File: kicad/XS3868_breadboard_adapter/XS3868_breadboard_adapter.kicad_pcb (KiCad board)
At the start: 2 copper layers, 26.4 x 31.5 mm, 12 parts, among them J1 SCJ368R1NUS0B00G, P1 CONN_01X12, P2 CONN_01X12, U1 XS3868

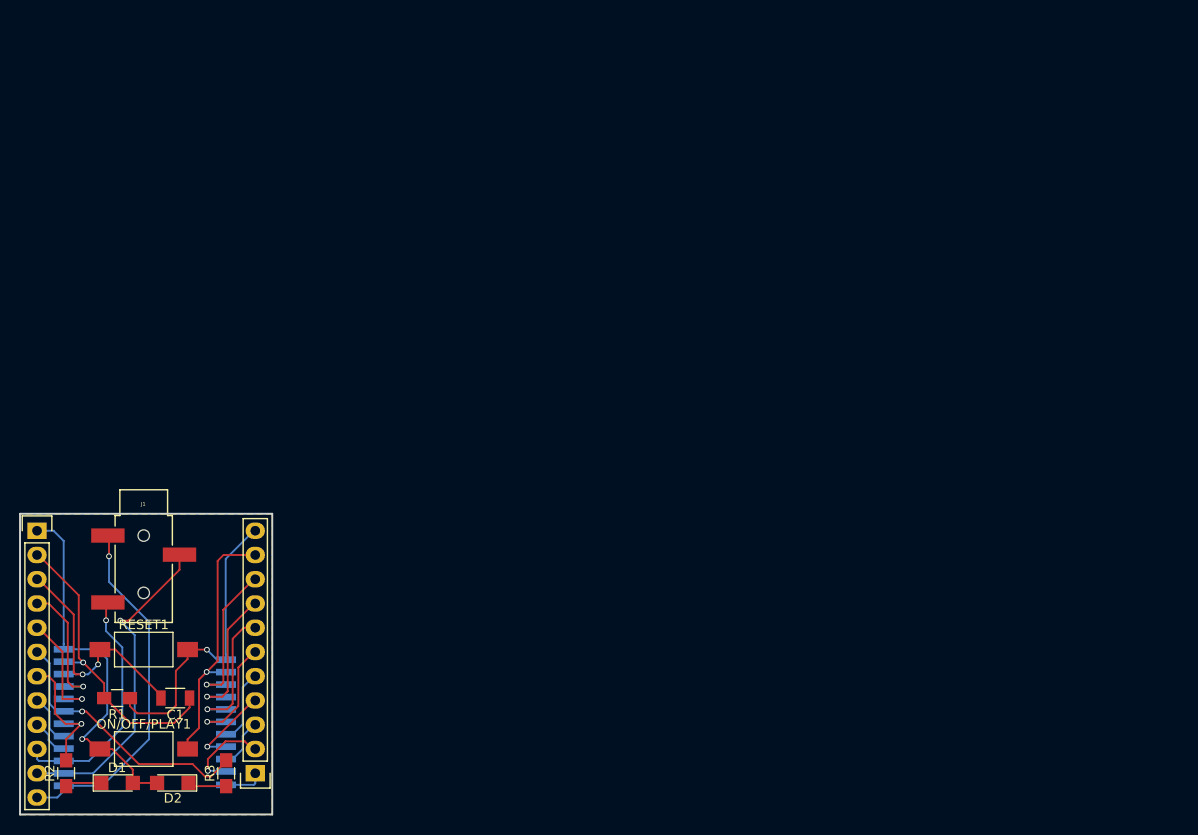
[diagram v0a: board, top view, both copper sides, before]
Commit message: update
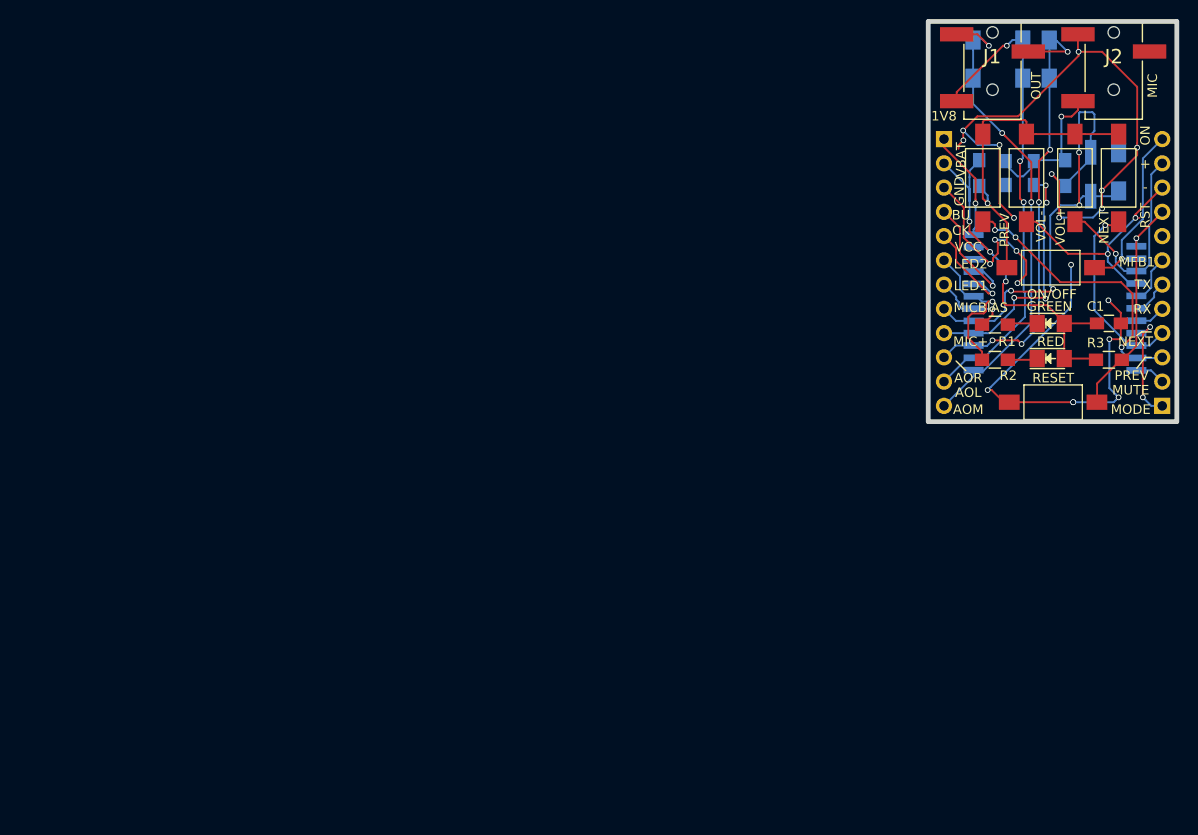
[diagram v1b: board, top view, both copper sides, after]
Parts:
- removed D1, D2: LED, LEDs:LED_1206
- removed ON/OFF/PLAY1: ON/OFF, Buttons_Switches_SMD:SW_SPST_FSMSM
- removed RESET1: 1, Buttons_Switches_SMD:SW_SPST_FSMSM
- added C2: 4u7, Capacitors_SMD.pretty:C_1206_HandSoldering, B.Cu at (164.1, 84.3)
- added C3: 2u2/6.5V, Capacitors_SMD.pretty:C_0805_HandSoldering, B.Cu at (155.2, 84.5)
- added C4: 220p/optional, Capacitors_SMD.pretty:C_0805_HandSoldering, B.Cu at (152.3, 84.5)
- added C5: 10uF, Capacitors_SMD.pretty:C_1206_HandSoldering, B.Cu at (148.8, 72.5)
- added C6: 10uF, Capacitors_SMD.pretty:C_1206_HandSoldering, B.Cu at (154.1, 72.5)
- added C7: 10uF, Capacitors_SMD.pretty:C_1206_HandSoldering, B.Cu at (156.8, 72.5)
- added GREEN: GREEN, LEDs:LED-1206, F.Cu at (157.0, 100.2)
- added J2: MIC, jacks:3.5mm_stereo_jack_PJ320B, F.Cu at (163.6, 69.7)
- added L1: 15n, Choke_SMD.pretty:Choke_SMD_1206_Handsoldering, B.Cu at (161.2, 84.6)
- added R4: 2k2, Resistors_SMD:R_0805_HandSoldering, B.Cu at (158.5, 84.5)
- added R5: 2k, Resistors_SMD:R_0805_HandSoldering, B.Cu at (149.5, 84.5)
- added RED: RED, LEDs:LED-1206, F.Cu at (157.0, 103.9)
- added SW1: PREV, Buttons_Switches_SMD:SW_SPST_FSMSM, F.Cu at (149.9, 85.0)
- added SW2: NEXT, Buttons_Switches_SMD:SW_SPST_FSMSM, F.Cu at (164.1, 85.0)
- added SW3: VOL-, Buttons_Switches_SMD:SW_SPST_FSMSM, F.Cu at (154.4, 85.0)
- added SW4: VOL+, Buttons_Switches_SMD:SW_SPST_FSMSM, F.Cu at (159.5, 85.0)
- added SW5: ON/OFF, Buttons_Switches_SMD:SW_SPST_FSMSM, F.Cu at (157.0, 94.4)
- added SW6: RESET, Buttons_Switches_SMD:SW_SPST_FSMSM, F.Cu at (157.2, 108.5)
- C1: footprint Capacitors_SMD:C_1206 -> Capacitors_SMD.pretty:C_0805_HandSoldering
- J1: value SCJ368R1NUS0B00G -> OUT
- P1: footprint Pin_Headers.pretty:Pin_Header_Straight_1x12 -> Pin_Headers:Pin_Header_Straight_1x12_Pitch2.54mm; moved to B.Cu
- P2: footprint Pin_Headers.pretty:Pin_Header_Straight_1x11 -> Pin_Headers:Pin_Header_Straight_1x12_Pitch2.54mm; moved to B.Cu
- R1: value 10k -> 470
- R3: value 470 -> 10k
- U1: footprint modules:XS3868 -> bluetooth:XS3868
- moved R2 106.5 mm to (151.1, 104.0), turned to 180 degrees
- moved C1 105.4 mm to (163.1, 100.2)
- moved U1 104.4 mm to (148.9, 89.6)
- moved P1 103.5 mm to (145.8, 80.9), turned to 180 degrees
- moved J1 103.3 mm to (150.9, 69.7)
- moved P2 102.5 mm to (168.7, 108.8), turned to 0 degrees
- moved R3 102.1 mm to (163.1, 104.0), turned to 180 degrees
- moved R1 99.9 mm to (151.1, 100.3)
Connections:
- net Net-(D1-Pad2) renamed /1V8
- net Net-(J1-Pad1) renamed /AOM
- net Net-(J1-Pad2) renamed /AOL
- net Net-(P1-Pad4) renamed /VBUCK
- net Net-(P1-Pad5) renamed /VCC
- net Net-(P1-Pad8) renamed /MICBIAS
- net Net-(P1-Pad9) renamed /MIC+
- net Net-(P2-Pad5) renamed /UART_RX
- net Net-(P2-Pad6) renamed /UART_TX
- net Net-(P2-Pad7) renamed /MFB1
- C1 pad 1: Net-(C1-Pad1) -> GND
- C1 pad 2: GND -> /VBAT
- P1 pad 10: Net-(J1-Pad5) -> /AOR
- P1 pad 2: Net-(C1-Pad1) -> /VBAT
- P1 pad 6: Net-(P1-Pad6) -> /LED2
- P1 pad 7: Net-(P1-Pad7) -> /LED1
- P2 pad 1: Net-(P2-Pad1) -> /MODE
- P2 pad 10: Net-(ON/OFF/PLAY1-Pad2) -> /VOL-
- P2 pad 11: Net-(P2-Pad11) -> /VOL+
- P2 pad 2: Net-(P2-Pad2) -> /MUTE
- P2 pad 3: Net-(P2-Pad3) -> /PREVIOUS
- P2 pad 4: Net-(P2-Pad4) -> /NEXT
- P2 pad 8: Net-(P2-Pad8) -> (no net)
- P2 pad 9: Net-(P2-Pad9) -> /RESET
- R1 pad 1: Net-(P2-Pad11) -> Net-(DG1-Pad1)
- R1 pad 2: Net-(C1-Pad1) -> /LED1
- R2 pad 2: Net-(P1-Pad7) -> /LED2
- R3 pad 1: Net-(D2-Pad1) -> /RESET
- R3 pad 2: Net-(P1-Pad6) -> /VBAT
- U1 pad 11: Net-(C1-Pad1) -> /VBAT
- U1 pad 13: Net-(P2-Pad11) -> /RESET
- U1 pad 14: Net-(ON/OFF/PLAY1-Pad2) -> /ONKEY
- U1 pad 15: Net-(P2-Pad9) -> /VOL+
- U1 pad 16: Net-(P2-Pad8) -> /VOL-
- U1 pad 20: Net-(P2-Pad4) -> /MODE
- U1 pad 21: Net-(P2-Pad3) -> /NEXT
- U1 pad 22: Net-(P2-Pad2) -> /PREVIOUS
- U1 pad 23: Net-(P2-Pad1) -> /MUTE
- U1 pad 3: Net-(J1-Pad5) -> /AOR
- U1 pad 6: Net-(P1-Pad7) -> /LED1
- U1 pad 7: Net-(P1-Pad6) -> /LED2
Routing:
- net GND: track 26.8 -> 129.2 mm, vias 2 -> 21
- net /AOR: track 0.00 -> 48.2 mm, vias 0 -> 5
- net /MICBIAS: track 5.39 -> 51.1 mm, vias 0 -> 4
- net /VBAT: track 0.00 -> 42.6 mm, vias 0 -> 3
- net Net-(R5-Pad2): track 0.00 -> 34.2 mm, vias 0 -> 1
- net Net-(P2-Pad11): track 32.0 -> 0.00 mm, vias 1 -> 0
- net Net-(C1-Pad1): track 31.8 -> 0.00 mm, vias 1 -> 0
- net /PREVIOUS: track 0.00 -> 30.9 mm, vias 0 -> 3
- net Net-(P1-Pad6): track 28.5 -> 0.00 mm, vias 1 -> 0
- net /1V8: track 39.6 -> 11.5 mm
- net Net-(ON/OFF/PLAY1-Pad2): track 27.2 -> 0.00 mm, vias 1 -> 0
- net Net-(J1-Pad5): track 25.4 -> 0.00 mm, vias 1 -> 0
- net /VOL-: track 0.00 -> 24.4 mm, vias 0 -> 2
- net /RESET: track 0.00 -> 23.7 mm, vias 0 -> 1
- net /MIC+: track 4.15 -> 27.6 mm, vias 0 -> 4
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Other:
- board size 26.4 x 31.5 mm -> 26 x 41.9 mm
- board text added: "+"
- board text added: "-"
- board text added: "1V8"
- board text added: "AOL"
- board text added: "AOM"
- board text added: "AOR"
- board text added: "BU CK"
- board text added: "GND"
- board text added: "LED1"
- board text added: "LED2"
- board text added: "MFB1"
- board text added: "MIC+"
- board text added: "MICBIAS"
- board text added: "MODE"
- board text added: "MUTE"
- board text added: "NEXT"
- board text added: "ON"
- board text added: "PREV"
- board text added: "RST"
- board text added: "RX"
- board text added: "TX"
- board text added: "VBAT"
- board text added: "VCC"
